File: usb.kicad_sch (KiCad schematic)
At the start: 5 parts, among them J1 TYPE-C-31-M-12, J3 USB_C_Receptacle_PowerOnly_6P

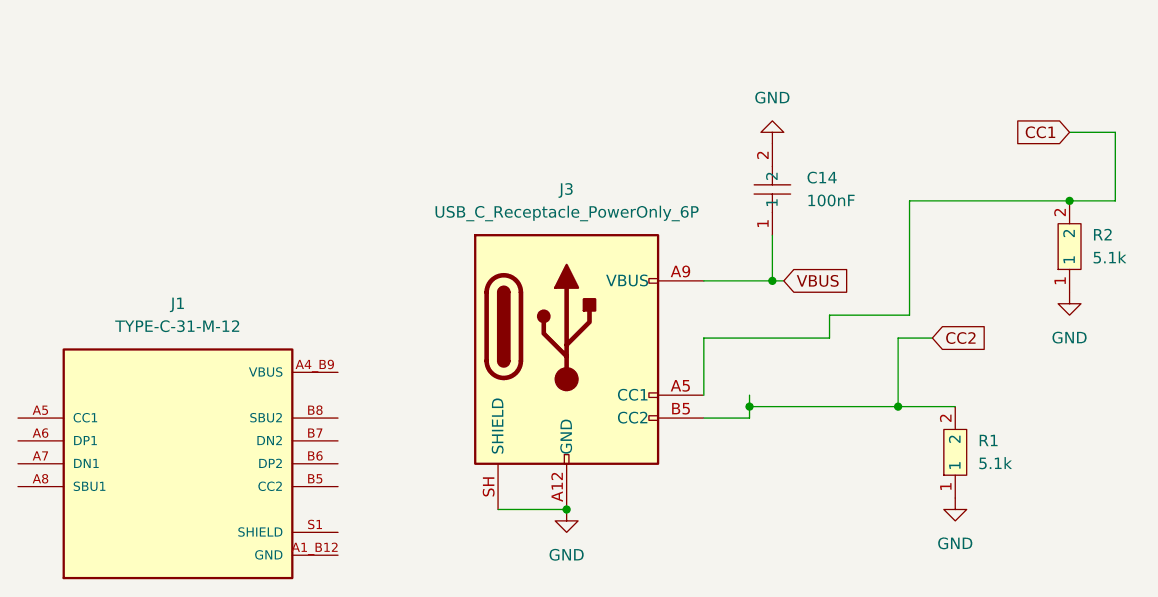
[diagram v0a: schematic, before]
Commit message: Update KiCad schematic and PCB files
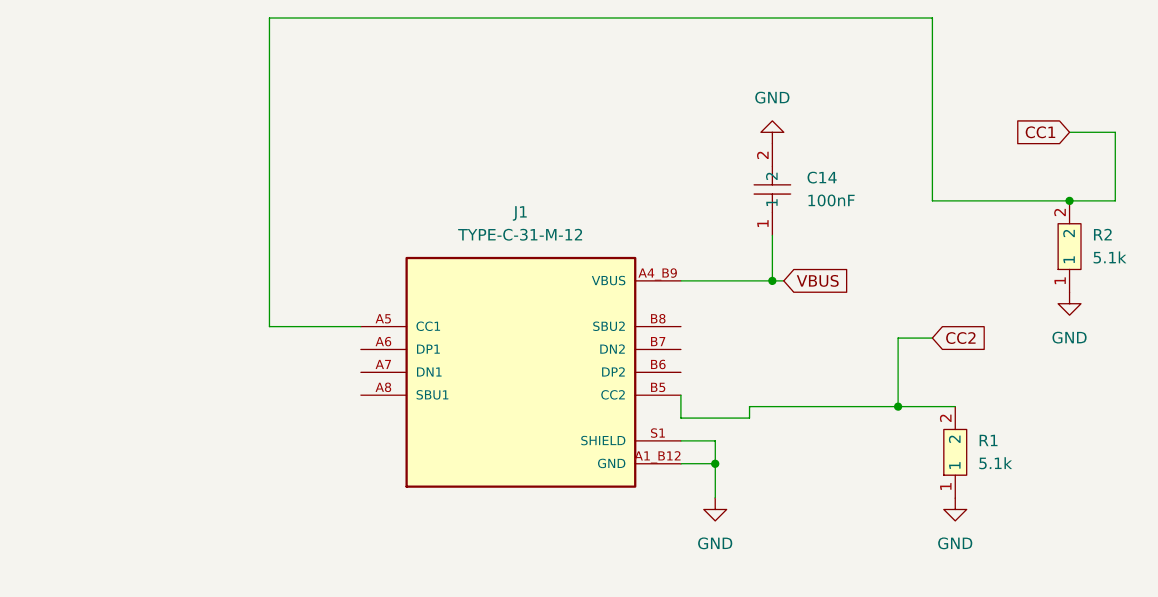
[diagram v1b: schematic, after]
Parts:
- removed J3: USB_C_Receptacle_PowerOnly_6P, Connector_USB:USB_C_Receptacle_HRO_TYPE-C-31-M-12, symbol Connector:USB_C_Receptacle_PowerOnly_6P
- J1: footprint TYPE-C-31-M-12:HRO_TYPE-C-31-M-12 -> easyeda2kicad:USB-C_SMD-TYPE-C-31-M-12_1
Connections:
- net CC1: now also J1.A5 (CC1)
- net CC2: now also J1.B5 (CC2)
- net GND: now also J1.S1 (SHIELD), J1.S2 (SHIELD), J1.S3 (SHIELD), J1.S4 (SHIELD)
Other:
- moved on the sheet: J1
